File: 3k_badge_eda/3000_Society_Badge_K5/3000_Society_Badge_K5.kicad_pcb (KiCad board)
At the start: 2 copper layers, 195.2 x 165.9 mm, 6 parts, among them IC1 Trinket_M0

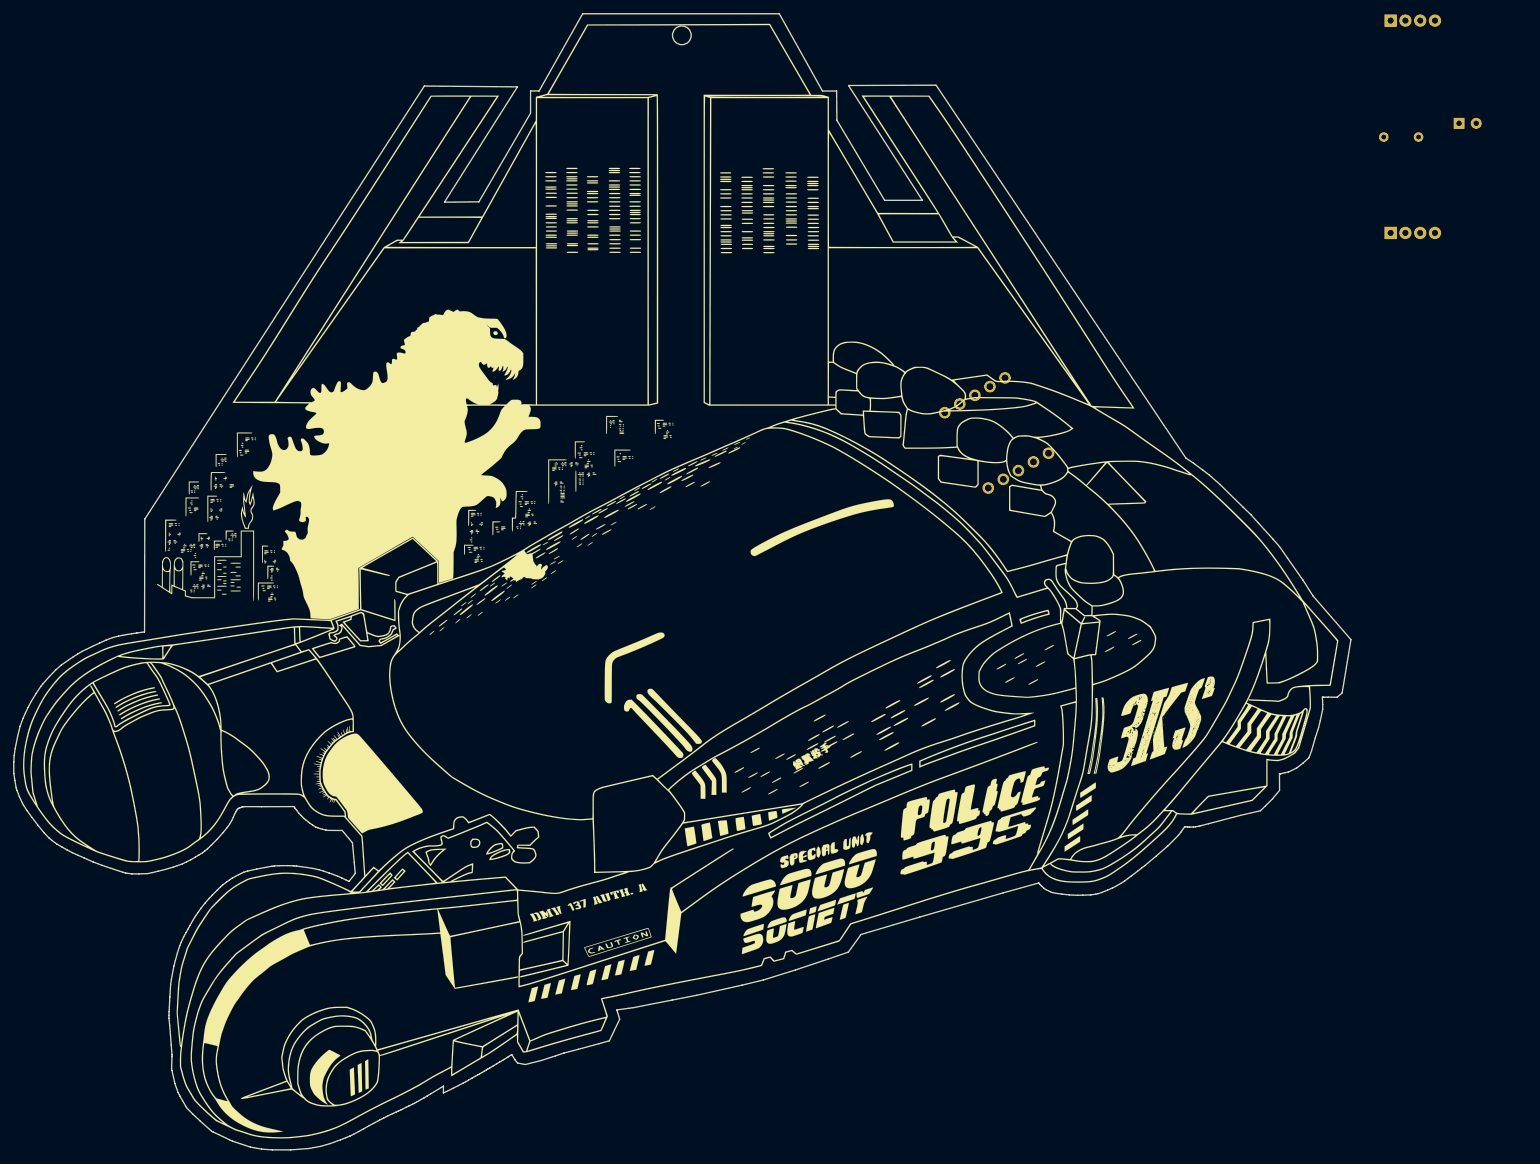
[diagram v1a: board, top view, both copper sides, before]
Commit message: PCB-updates
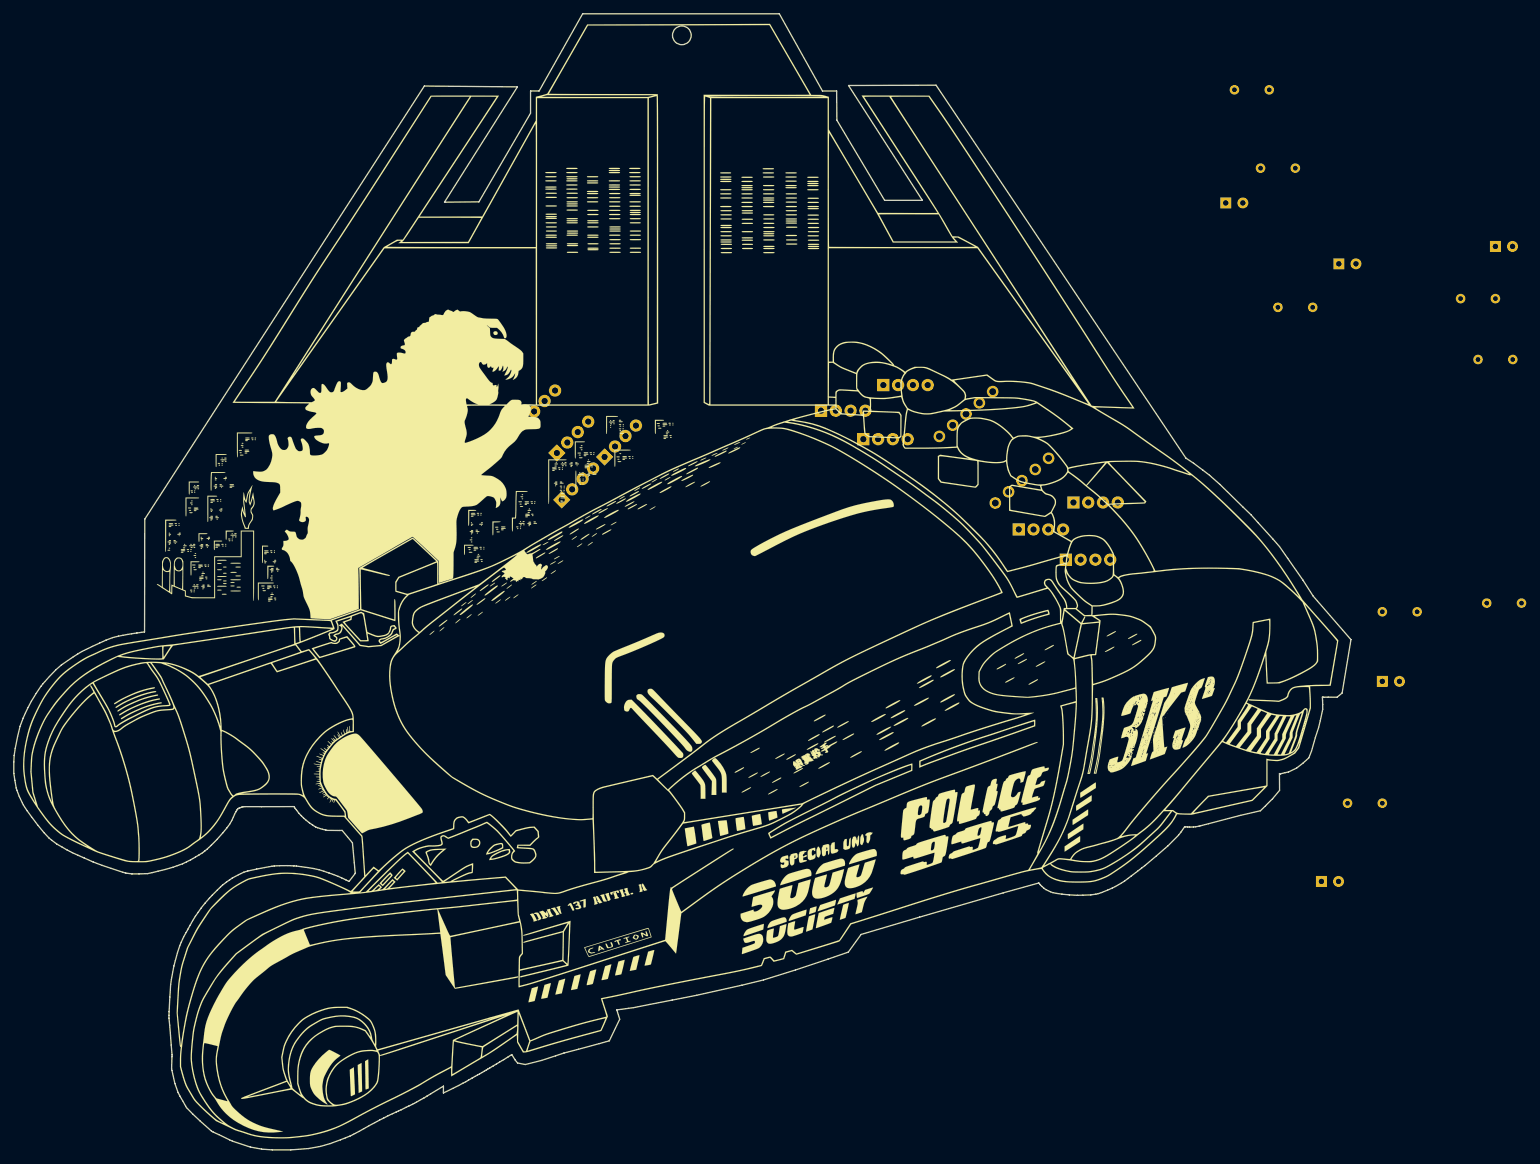
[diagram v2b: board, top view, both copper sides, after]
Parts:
- removed C1: CP 100uf, 3000_Society_Badge:CP_Radial_D6.3mm_P2.50mm
- removed D1: LED_NeoPixel_THT_5mm, 3000_Society_Badge:LED_D5.0mm-4_RGB_Wide_Pins
- removed D2: LED_NeoPixel_THT_8mm, 3000_Society_Badge:LED_D8.0mm-4_RGB
- removed R1: R 220ohm, 3000_Society_Badge:R_Axial_DIN0204_L3.6mm_D1.6mm_P5.08mm_Horizontal
- added C01: CP 100uF, 3000_Society_Badge:CP_Radial_D6.3mm_P2.50mm, F.Cu at (243.8, 118.1)
- added C02: CP 100uF, 3000_Society_Badge:CP_Radial_D6.3mm_P2.50mm, F.Cu at (234.9, 147.3)
- added C03: CP 100uF, 3000_Society_Badge:CP_Radial_D6.3mm_P2.50mm, F.Cu at (237.5, 57.1)
- added C04: CP 100uF, 3000_Society_Badge:CP_Radial_D6.3mm_P2.50mm, F.Cu at (260.4, 54.6)
- added C05: CP 100uF, 3000_Society_Badge:CP_Radial_D6.3mm_P2.50mm, F.Cu at (221.0, 48.3)
- added D10: LED_NeoPixel_THT_5mm, 3000_Society_Badge:LED_D5.0mm-4_RGB_Wide_Pins, F.Cu at (118.5, 80.2)
- added D11: LED_NeoPixel_THT_5mm, 3000_Society_Badge:LED_D5.0mm-4_RGB_Wide_Pins, F.Cu at (123.3, 84.8)
- added D12: LED_NeoPixel_THT_5mm, 3000_Society_Badge:LED_D5.0mm-4_RGB_Wide_Pins, F.Cu at (130.3, 85.3)
- added D13: LED_NeoPixel_THT_5mm, 3000_Society_Badge:LED_D5.0mm-4_RGB_Wide_Pins, F.Cu at (124.0, 91.6)
- added D20: LED_NeoPixel_THT_8mm, 3000_Society_Badge:LED_D8.0mm-4_RGB, F.Cu at (198.7, 92.0)
- added D21: LED_NeoPixel_THT_5mm, 3000_Society_Badge:LED_D5.0mm-4_RGB_Wide_Pins, F.Cu at (190.8, 95.9)
- added D22: LED_NeoPixel_THT_5mm, 3000_Society_Badge:LED_D5.0mm-4_RGB_Wide_Pins, F.Cu at (197.6, 100.3)
- added D40: LED_NeoPixel_THT_8mm, 3000_Society_Badge:LED_D8.0mm-4_RGB, F.Cu at (171.0, 74.9)
- added D41: LED_NeoPixel_THT_5mm, 3000_Society_Badge:LED_D5.0mm-4_RGB_Wide_Pins, F.Cu at (161.9, 78.6)
- added D42: LED_NeoPixel_THT_5mm, 3000_Society_Badge:LED_D5.0mm-4_RGB_Wide_Pins, F.Cu at (168.1, 82.8)
- added R01: R 470ohm, 3000_Society_Badge:R_Axial_DIN0204_L3.6mm_D1.6mm_P5.08mm_Horizontal, F.Cu at (243.8, 108.0)
- added R02: R 470ohm, 3000_Society_Badge:R_Axial_DIN0204_L3.6mm_D1.6mm_P5.08mm_Horizontal, F.Cu at (238.8, 135.9)
- added R03: R 470ohm, 3000_Society_Badge:R_Axial_DIN0204_L3.6mm_D1.6mm_P5.08mm_Horizontal, F.Cu at (228.6, 63.5)
- added R04: R 470ohm, 3000_Society_Badge:R_Axial_DIN0204_L3.6mm_D1.6mm_P5.08mm_Horizontal, F.Cu at (255.3, 62.2)
- added R05: R 470ohm, 3000_Society_Badge:R_Axial_DIN0204_L3.6mm_D1.6mm_P5.08mm_Horizontal, F.Cu at (226.1, 43.2)
- added R10: R 470ohm, 3000_Society_Badge:R_Axial_DIN0204_L3.6mm_D1.6mm_P5.08mm_Horizontal, F.Cu at (259.1, 106.7)
- added R20: R 470ohm, 3000_Society_Badge:R_Axial_DIN0204_L3.6mm_D1.6mm_P5.08mm_Horizontal, F.Cu at (257.8, 71.1)
- added R40: R 470ohm, 3000_Society_Badge:R_Axial_DIN0204_L3.6mm_D1.6mm_P5.08mm_Horizontal, F.Cu at (222.2, 31.8)
- moved IC1 1.79 mm to (197.8, 75.0), turned to 310 degrees
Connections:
- IC1 pad 10: (no net) -> Net-(IC1-Pad10)
- IC1 pad 2: (no net) -> Net-(C01-Pad2)
- IC1 pad 3: (no net) -> Net-(IC1-Pad3)
- IC1 pad 7: (no net) -> Net-(IC1-Pad7)
- IC1 pad 8: (no net) -> Net-(IC1-Pad8)
